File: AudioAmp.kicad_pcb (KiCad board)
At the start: 2 copper layers, 130 x 85 mm, 67 parts, among them J1 Conn_01x01, J2 Conn_01x01, J3 Conn_01x01, J4 Conn_01x01, J5 Conn_01x01, Q1 2N5401, Q10 2SD669, Q11 2SD669, Q12 2N5551, Q13 2N5401, Q14 2SD669, Q15 2SB649, Q16 2SA1302, Q17 2SC3281, Q2 2N5551, Q3 2N5401, Q4 2N5551, Q5 2N5401, Q6 2N5401, Q7 2N5551, Q8 2SD669, Q9 2SB649

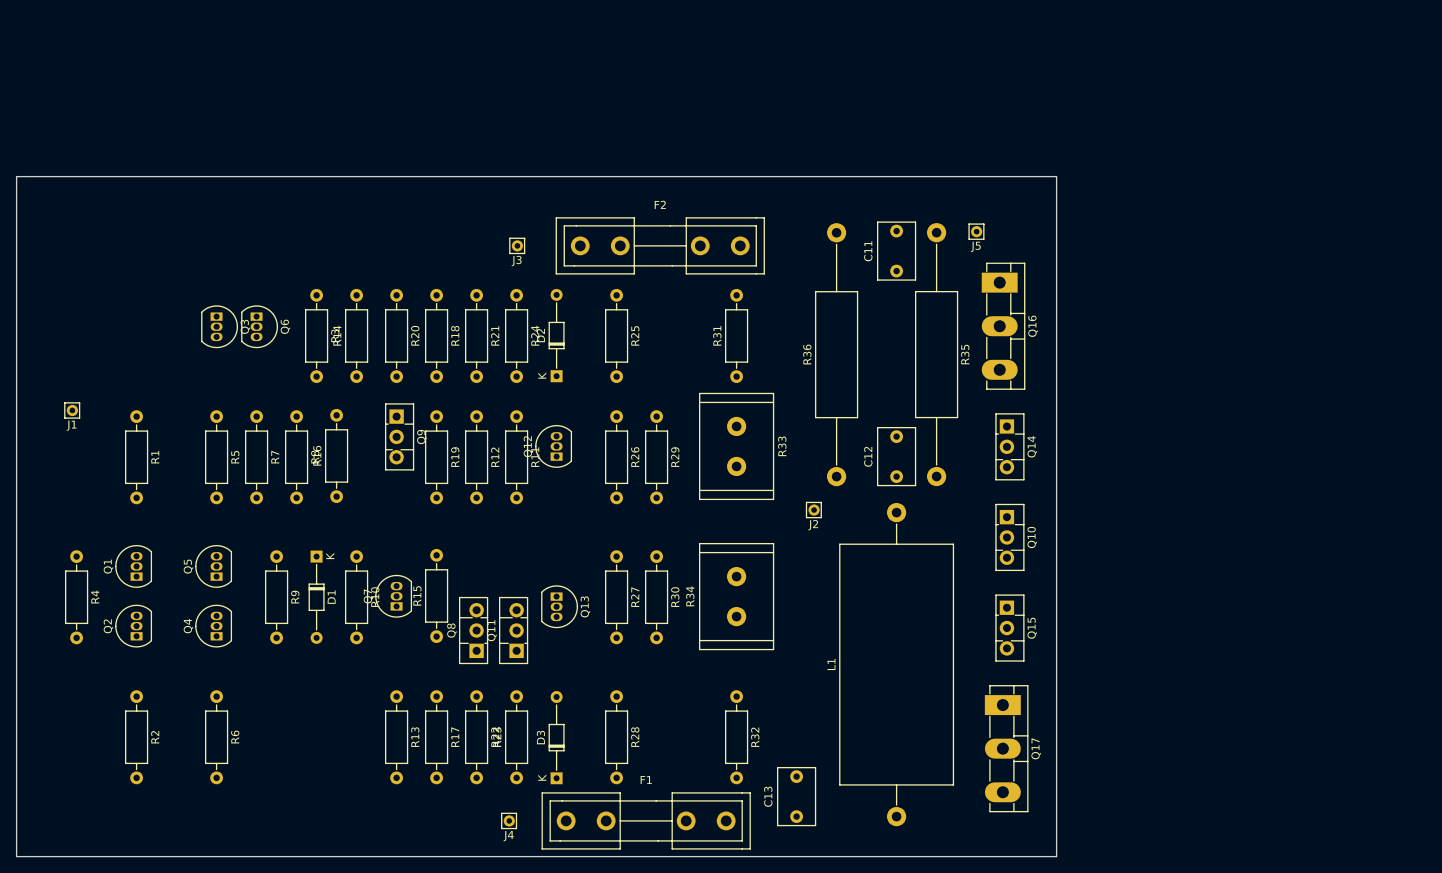
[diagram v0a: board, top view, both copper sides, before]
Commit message: placement done
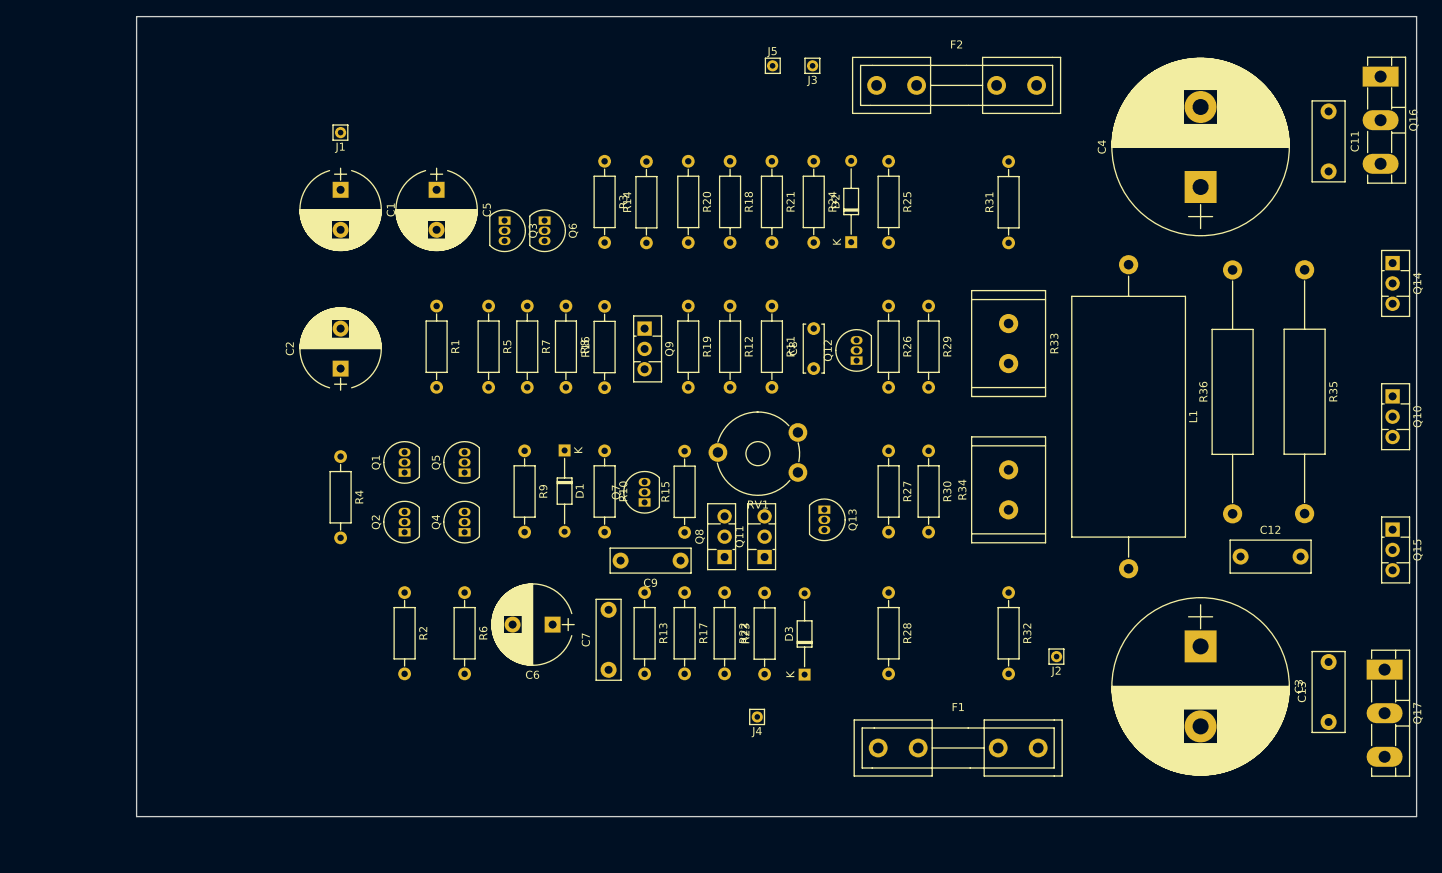
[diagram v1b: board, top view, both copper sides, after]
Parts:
- added C1: 47u, Capacitors_THT:CP_Radial_D10.0mm_P5.00mm, F.Cu at (95.5, 66.7)
- added C2: 47u, Capacitors_THT:CP_Radial_D10.0mm_P5.00mm, F.Cu at (95.5, 89.0)
- added C3: 220u, Capacitors_THT:CP_Radial_D22.0mm_P10.00mm_SnapIn, F.Cu at (203.0, 123.7)
- added C4: 220u, Capacitors_THT:CP_Radial_D22.0mm_P10.00mm_SnapIn, F.Cu at (203.0, 66.3)
- added C5: 47u, Capacitors_THT:CP_Radial_D10.0mm_P5.00mm, F.Cu at (107.5, 66.7)
- added C6: 220u, Capacitors_THT:CP_Radial_D10.0mm_P5.00mm, F.Cu at (122.0, 121.0)
- added C7: 150p, Capacitors_THT:C_Rect_L10.0mm_W3.0mm_P7.50mm_MKS4, F.Cu at (129.0, 126.7)
- added C8: 5p, Capacitors_THT:C_Disc_D6.0mm_W2.5mm_P5.00mm, F.Cu at (154.6, 89.0)
- added C9: 300p, Capacitors_THT:C_Rect_L10.0mm_W3.0mm_P7.50mm_MKS4, F.Cu at (138.0, 113.0)
- added RV1: 1K, Potentiometers:Potentiometer_Trimmer_Piher_PT-10v10_Horizontal_Px10.0mm_Py5.0mm, F.Cu at (152.7, 97.0)
- C11, C12, C13: footprint Capacitor_THT:C_Rect_L7.0mm_W4.5mm_P5.00mm -> Capacitors_THT:C_Rect_L10.0mm_W4.0mm_P7.50mm_MKS4
- R1, R10, R11, R12, R13, R14, R15, R16, R17, R18, R19, R2, R20, R21, R22, R23, R24, R25, R26, R27, R28, R29, R3, R30, R31, R32, R4, R5, R6, R7, R8, R9: footprint Resistor_THT:R_Axial_DIN0207_L6.3mm_D2.5mm_P10.16mm_Horizontal -> Resistors_THT:R_Axial_DIN0207_L6.3mm_D2.5mm_P10.16mm_Horizontal
- R35, R36: footprint Resistor_THT:R_Axial_DIN0516_L15.5mm_D5.0mm_P30.48mm_Horizontal -> Resistors_THT:R_Axial_DIN0516_L15.5mm_D5.0mm_P30.48mm_Horizontal
- moved L1 74.8 mm to (194.0, 76.0), turned to 270 degrees
- moved C13 67.5 mm to (219.0, 133.2)
- moved C11 57.6 mm to (219.0, 56.9), turned to 270 degrees
- moved Q16 54.1 mm to (225.5, 52.5)
- moved Q14 52.4 mm to (227.0, 75.8)
- moved Q10 50.5 mm to (227.0, 92.5)
- moved R36 49.7 mm to (207.0, 107.2)
- moved Q15 49.2 mm to (227.0, 109.1)
- moved J1 48.3 mm to (95.5, 59.5)
- moved Q17 47.9 mm to (226.0, 126.6)
- moved R35 46.2 mm to (216.0, 76.7)
- moved C12 44.1 mm to (208.0, 112.5), turned to 0 degrees
- moved J3 43.2 mm to (154.5, 51.1)
- moved F2 42.1 mm to (162.5, 53.6)
- moved R24 40.7 mm to (154.6, 63.1)
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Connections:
- net Net-(C11-Pad2) renamed /VCC_FUSED
- net Net-(C13-Pad1) renamed /VSS_FUSED
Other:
- board size 130 x 85 mm -> 160 x 100 mm
- net class HIGH_CURRENT added: clearance 0.5, trace_width 1, via_dia 0.8, via_drill 0.4
